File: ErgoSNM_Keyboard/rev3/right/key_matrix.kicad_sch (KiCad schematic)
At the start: 58 parts

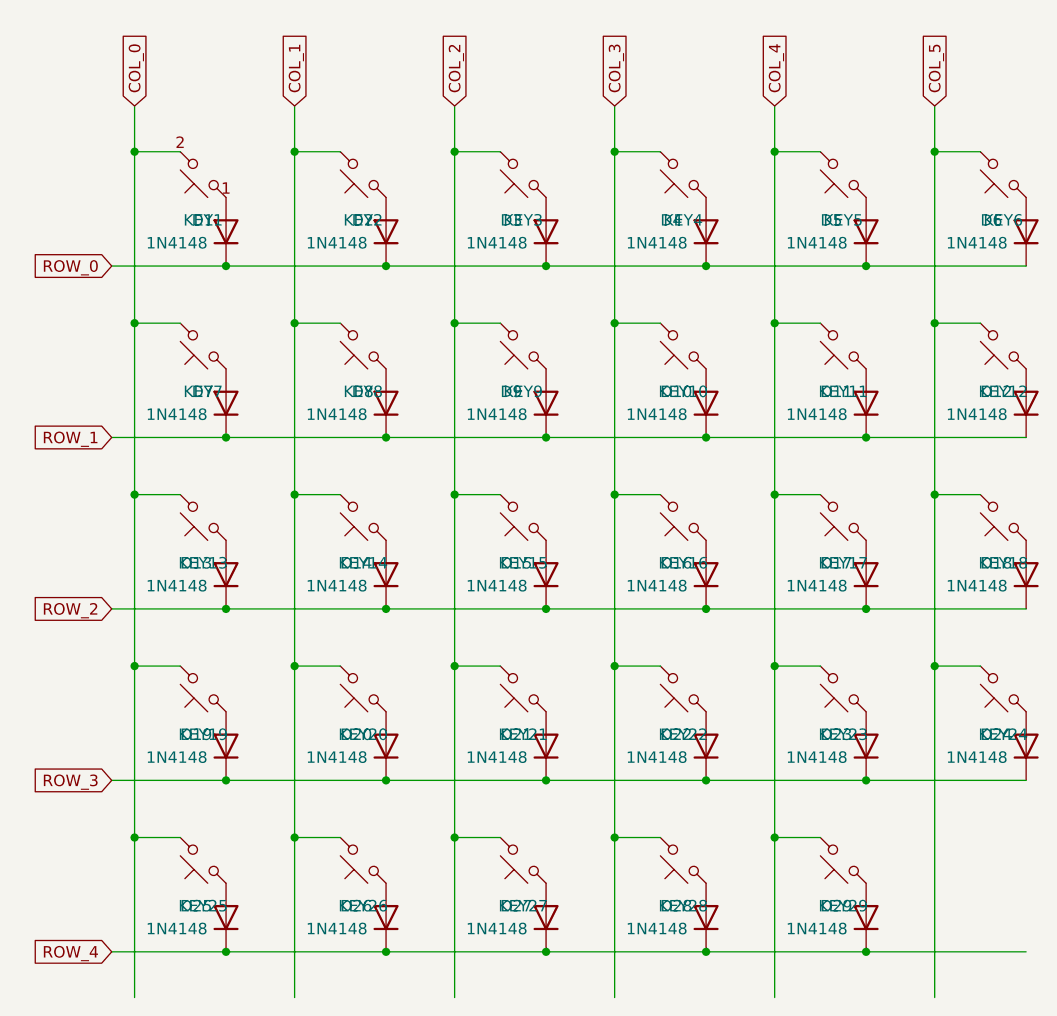
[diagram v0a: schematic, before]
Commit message: Update submodule
Update submodule

Update switch footprint
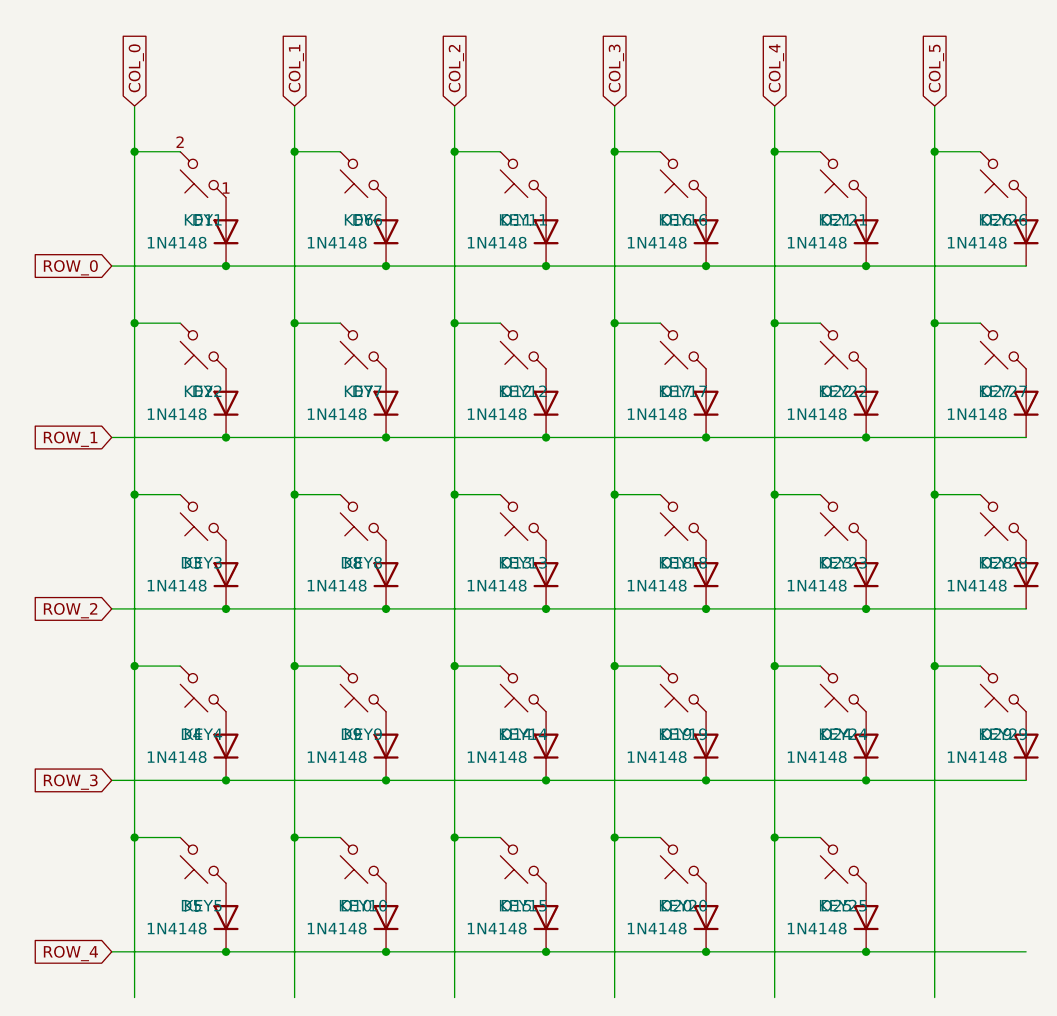
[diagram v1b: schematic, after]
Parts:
- renumbered D26 to D10, D3 to D11, D9 to D12, D15 to D13, D21 to D14, D27 to D15, D4 to D16, D10 to D17, D16 to D18, D22 to D19, D7 to D2, D28 to D20, D5 to D21, D11 to D22, D17 to D23, D23 to D24, D29 to D25, D6 to D26, D12 to D27, D18 to D28, D24 to D29, D13 to D3, D19 to D4, D25 to D5, D2 to D6, D8 to D7, D14 to D8, D20 to D9, KEY26 to KEY10, KEY3 to KEY11, KEY9 to KEY12, KEY15 to KEY13, KEY21 to KEY14, KEY27 to KEY15, KEY4 to KEY16, KEY10 to KEY17, KEY16 to KEY18, KEY22 to KEY19, KEY7 to KEY2, KEY28 to KEY20, KEY5 to KEY21, KEY11 to KEY22, KEY17 to KEY23, KEY23 to KEY24, KEY29 to KEY25, KEY6 to KEY26, KEY12 to KEY27, KEY18 to KEY28, KEY24 to KEY29, KEY13 to KEY3, KEY19 to KEY4, KEY25 to KEY5, KEY2 to KEY6, KEY8 to KEY7, KEY14 to KEY8, KEY20 to KEY9
